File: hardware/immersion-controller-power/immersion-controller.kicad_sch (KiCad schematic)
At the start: 1 part, among them J1 MCU

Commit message: debugged prototype
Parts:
- J1: footprint Connector_PinHeader_1.27mm:PinHeader_1x04_P1.27mm_Horizontal -> Connector_PinHeader_2.54mm:PinHeader_1x04_P2.54mm_Vertical
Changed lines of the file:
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@@
       (effects (font (size 1.27 1.27)))
     )
-    (property "Footprint" "Connector_PinHeader_1.27mm:PinHeader_1x04_P1.27mm_Horizontal" (at 156.464 52.07 0)
+    (property "Footprint" "Connector_PinHeader_2.54mm:PinHeader_1x04_P2.54mm_Vertical" (at 156.464 52.07 0)
       (effects (font (size 1.27 1.27)) hide)
     )

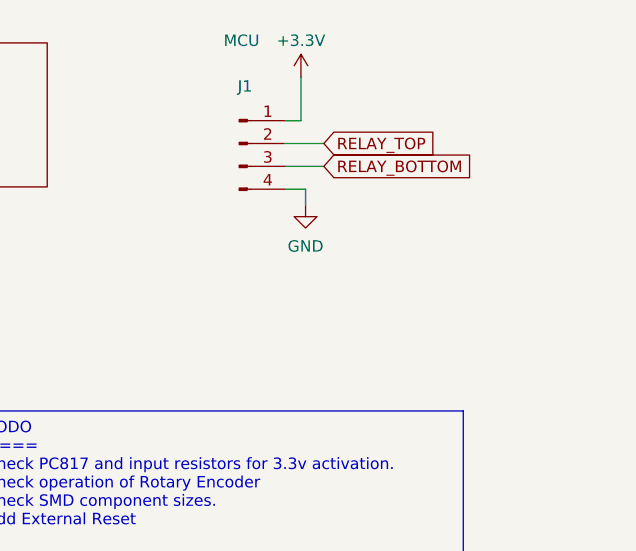
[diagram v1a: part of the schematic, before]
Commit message: Initial Prototype results
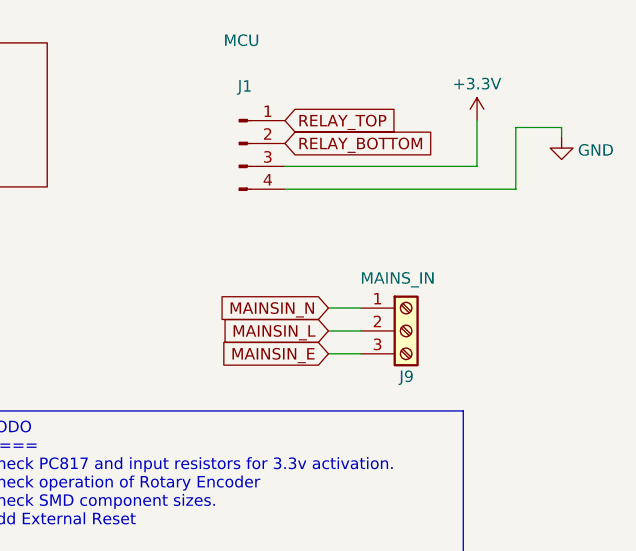
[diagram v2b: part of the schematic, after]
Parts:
- added J9: MAINS_IN, TerminalBlock_Dinkle:TerminalBlock_Dinkle_DT-55-B01X-03_P10.00mm, symbol Connector:Screw_Terminal_01x03
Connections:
- net +3.3V: now also J1.3 (Pin_3); no longer J1.1 (Pin_1)
- net RELAY_BOTTOM: now also J1.2 (Pin_2); no longer J1.3 (Pin_3)
- net RELAY_TOP: now also J1.1 (Pin_1); no longer J1.2 (Pin_2)
- new net MAINSIN_E: J9.3 (Pin_3)
- new net MAINSIN_L: J9.2 (Pin_2)
- new net MAINSIN_N: J9.1 (Pin_1)
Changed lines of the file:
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@@
 (kicad_sch (version 20230121) (generator eeschema)
   (paper "A4")
-  (wire (pts (xy 163.83 57.15) (xy 163.83 58.928))
+  (wire (pts (xy 166.37 70.358) (xy 169.926 70.358))
     (stroke (width 0) (type default))
   )
-  (wire (pts (xy 161.544 54.61) (xy 165.862 54.61))
+  (wire (pts (xy 166.37 72.898) (xy 169.926 72.898))
     (stroke (width 0) (type default))
   )
-  (wire (pts (xy 163.322 49.53) (xy 161.544 49.53))
+  (wire (pts (xy 161.544 57.15) (xy 187.198 57.15))
     (stroke (width 0) (type default))
   )
-  (wire (pts (xy 163.322 44.704) (xy 163.322 49.53))
+  (wire (pts (xy 161.544 54.61) (xy 182.88 54.61))
     (stroke (width 0) (type default))
   )
-  (wire (pts (xy 161.544 52.07) (xy 165.862 52.07))
+  (wire (pts (xy 192.278 50.292) (xy 192.278 51.308))
     (stroke (width 0) (type default))
   )
-  (wire (pts (xy 161.544 57.15) (xy 163.83 57.15))
+  (wire (pts (xy 166.37 75.438) (xy 169.926 75.438))
+    (stroke (width 0) (type default))
+  )
+  (wire (pts (xy 187.198 50.292) (xy 187.198 57.15))
+    (stroke (width 0) (type default))
+  )
+  (wire (pts (xy 182.88 49.53) (xy 182.88 54.61))
+    (stroke (width 0) (type default))
+  )
+  (wire (pts (xy 187.198 50.292) (xy 192.278 50.292))
     (stroke (width 0) (type default))
   )
@@
     (effects (font (size 1.27 1.27)) (justify left top))
   )
-  (global_label "RELAY_TOP" (shape input) (at 165.862 52.07 0) (fields_autoplaced)
+  (global_label "RELAY_BOTTOM" (shape input) (at 161.544 52.07 0) (fields_autoplaced)
     (effects (font (size 1.27 1.27)) (justify left))
-    (property "Intersheetrefs" "${INTERSHEET_REFS}" (at 178.9278 52.07 0)
+    (property "Intersheetrefs" "${INTERSHEET_REFS}" (at 178.4387 52.07 0)
       (effects (font (size 1.27 1.27)) (justify left) hide)
     )
   )
-  (global_label "RELAY_BOTTOM" (shape input) (at 165.862 54.61 0) (fields_autoplaced)
+  (global_label "MAINSIN_E" (shape input) (at 166.37 75.438 180) (fields_autoplaced)
+    (effects (font (size 1.27 1.27)) (justify right))
+    (property "Intersheetrefs" "${INTERSHEET_REFS}" (at 153.7275 75.438 0)
+      (effects (font (size 1.27 1.27)) (justify right) hide)
+    )
+  )
+  (global_label "MAINSIN_L" (shape input) (at 166.37 72.898 180) (fields_autoplaced)
+    (effects (font (size 1.27 1.27)) (justify right))
+    (property "Intersheetrefs" "${INTERSHEET_REFS}" (at 153.8484 72.898 0)
+      (effects (font (size 1.27 1.27)) (justify right) hide)
+    )
+  )
+  (global_label "RELAY_TOP" (shape input) (at 161.544 49.53 0) (fields_autoplaced)
     (effects (font (size 1.27 1.27)) (justify left))
-    (property "Intersheetrefs" "${INTERSHEET_REFS}" (at 182.6773 54.61 0)
+    (property "Intersheetrefs" "${INTERSHEET_REFS}" (at 174.6892 49.53 0)
       (effects (font (size 1.27 1.27)) (justify left) hide)
     )
   )
-  (symbol (lib_id "power:GND") (at 163.83 58.928 0) (unit 1)
-    (in_bom yes) (on_board yes) (dnp no) (fields_autoplaced)
-    (property "Reference" "#PWR04" (at 163.83 65.278 0)
+  (global_label "MAINSIN_N" (shape input) (at 166.37 70.358 180) (fields_autoplaced)
+    (effects (font (size 1.27 1.27)) (justify right))
+    (property "Intersheetrefs" "${INTERSHEET_REFS}" (at 153.546 70.358 0)
+      (effects (font (size 1.27 1.27)) (justify right) hide)
+    )
+  )
+  (symbol (lib_id "power:GND") (at 192.278 51.308 0) (unit 1)
+    (in_bom yes) (on_board yes) (dnp no)
+    (property "Reference" "#PWR04" (at 192.278 57.658 0)
       (effects (font (size 1.27 1.27)) hide)
     )
-    (property "Value" "GND" (at 163.83 63.5 0)
+    (property "Value" "GND" (at 196.088 52.832 0)
       (effects (font (size 1.27 1.27)))
     )
-    (property "Footprint" "" (at 163.83 58.928 0)
+    (property "Footprint" "" (at 192.278 51.308 0)
       (effects (font (size 1.27 1.27)) hide)
     )
-    (property "Datasheet" "" (at 163.83 58.928 0)
+    (property "Datasheet" "" (at 192.278 51.308 0)
       (effects (font (size 1.27 1.27)) hide)
     )
@@
     )
   )
-  (symbol (lib_id "power:+3.3V") (at 163.322 44.704 0) (unit 1)
-    (in_bom yes) (on_board yes) (dnp no) (fields_autoplaced)
-    (property "Reference" "#PWR05" (at 163.322 48.514 0)
+  (symbol (lib_id "Connector:Screw_Terminal_01x03") (at 175.006 72.898 0) (unit 1)
+    (in_bom yes) (on_board yes) (dnp no)
+    (property "Reference" "J9" (at 174.244 77.978 0)
+      (effects (font (size 1.27 1.27)) (justify left))
+    )
+    (property "Value" "MAINS_IN" (at 169.926 67.056 0)
+      (effects (font (size 1.27 1.27)) (justify left))
+    )
+    (property "Footprint" "TerminalBlock_Dinkle:TerminalBlock_Dinkle_DT-55-B01X-03_P10.00mm" (at 175.006 72.898 0)
       (effects (font (size 1.27 1.27)) hide)
     )
-    (property "Value" "+3.3V" (at 163.322 40.64 0)
+    (property "Datasheet" "~" (at 175.006 72.898 0)
+      (effects (font (size 1.27 1.27)) hide)
+    )
+    (pin "1")
+    (pin "2")
+    (pin "3")
+    (instances
+      (project "immersion-controller"
+        (path "/bd6e6743-d7bb-4018-a688-d589a8d21d49/bc36bd11-3fe8-4335-9c44-42b1c7dd4ff6"
+          (reference "J9") (unit 1)
+        )
+        (path "/bd6e6743-d7bb-4018-a688-d589a8d21d49"
+          (reference "J2") (unit 1)
+        )
+      )
+    )
+  )
+  (symbol (lib_id "power:+3.3V") (at 182.88 49.53 0) (unit 1)
+    (in_bom yes) (on_board yes) (dnp no) (fields_autoplaced)
+    (property "Reference" "#PWR05" (at 182.88 53.34 0)
+      (effects (font (size 1.27 1.27)) hide)
+    )
+    (property "Value" "+3.3V" (at 182.88 45.466 0)
       (effects (font (size 1.27 1.27)))
     )
-    (property "Footprint" "" (at 163.322 44.704 0)
+    (property "Footprint" "" (at 182.88 49.53 0)
       (effects (font (size 1.27 1.27)) hide)
     )
-    (property "Datasheet" "" (at 163.322 44.704 0)
+    (property "Datasheet" "" (at 182.88 49.53 0)
       (effects (font (size 1.27 1.27)) hide)
     )
